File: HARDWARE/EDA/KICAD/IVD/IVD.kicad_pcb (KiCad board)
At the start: 2 copper layers, 62 x 24 mm, 16 parts, among them J1 V_INPUT, J2 Digital_Info, Q1 BC549, U1 4N25

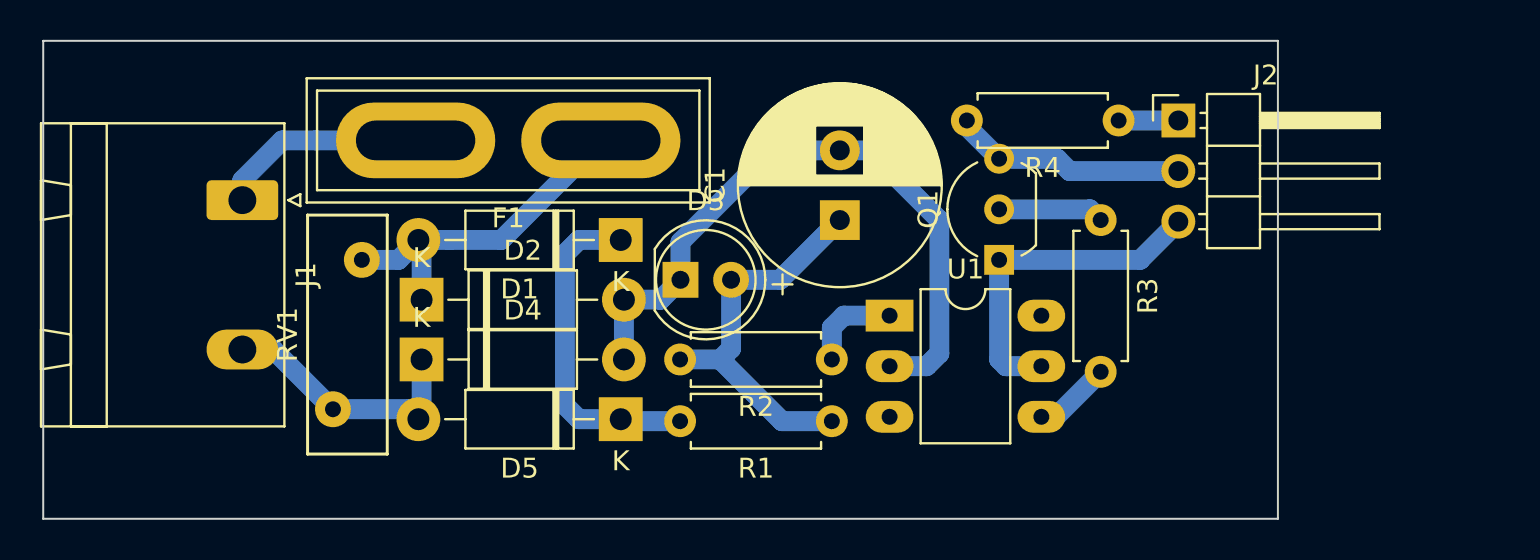
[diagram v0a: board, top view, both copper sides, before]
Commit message: finished board
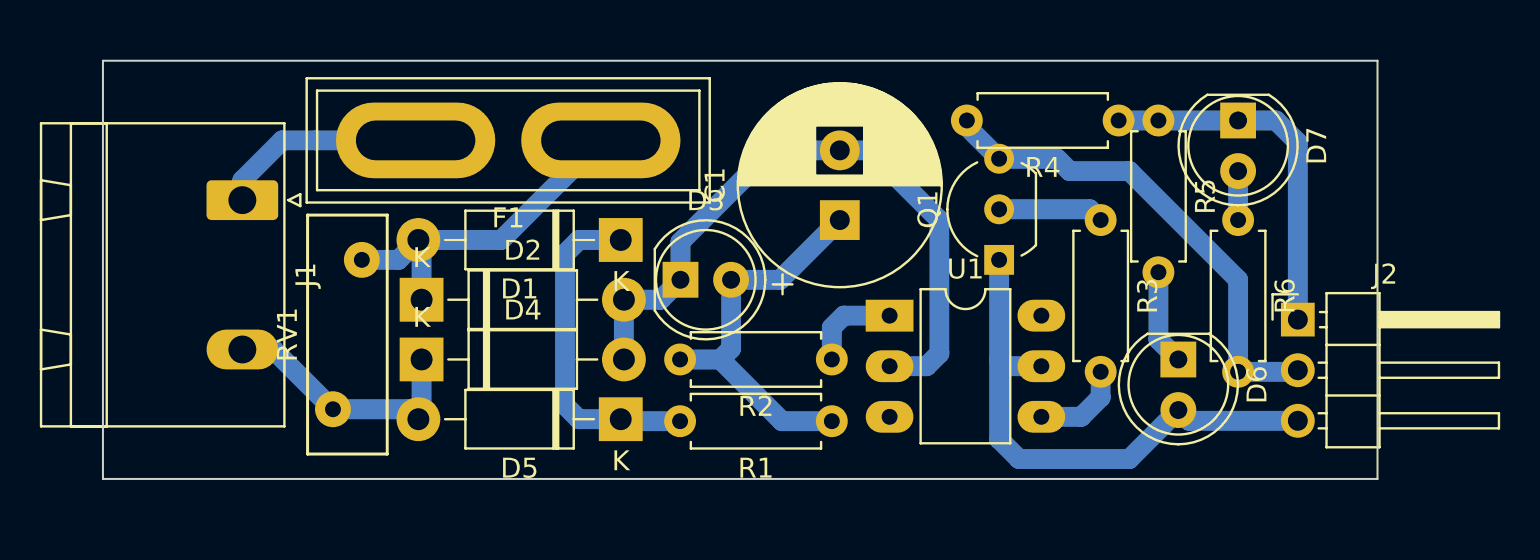
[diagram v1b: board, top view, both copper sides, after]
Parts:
- added D6: LED, LED_THT:LED_D5.0mm, F.Cu at (151.0, 85.0)
- added D7: LED, LED_THT:LED_D5.0mm_IRGrey, F.Cu at (154.0, 73.0)
- added R5: 100R, Resistor_THT:R_Axial_DIN0207_L6.3mm_D2.5mm_P7.62mm_Horizontal, F.Cu at (150.0, 73.0)
- added R6: 100R, Resistor_THT:R_Axial_DIN0207_L6.3mm_D2.5mm_P7.62mm_Horizontal, F.Cu at (154.0, 78.0)
- moved J2 11.7 mm to (157.0, 83.0)
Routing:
- net GNDD: track 3.00 -> 18.4 mm
- net V_Signal: track 11.8 -> 24.8 mm
- net +5VD: track 17.1 -> 27.9 mm
- net Net-(D6-Pad1): track 0.00 -> 4.79 mm
- net Net-(D7-Pad2): track 0.00 -> 2.46 mm
- net Net-(R3-Pad2): track 3.92 -> 4.67 mm
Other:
- board size 62 x 24 mm -> 64 x 21 mm
